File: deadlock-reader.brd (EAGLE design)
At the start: 49.2 x 49.5 mm, 49 parts, among them IC1 LM386M-1, IC2 STM32F072XX, IC3 MCP16301/H, IC4 MAX3232CSE, J1 RJ12 6p6c, X1 MINI-USB-SCHIELD-32005-301

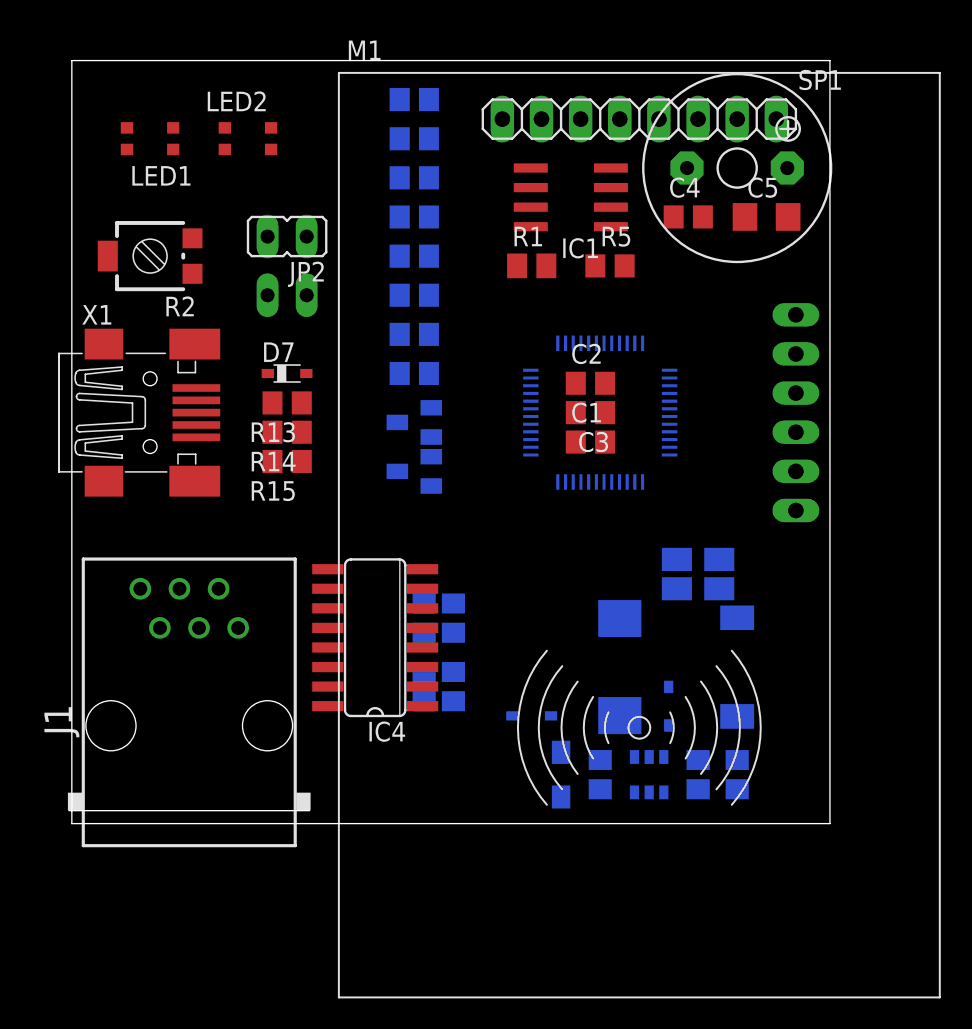
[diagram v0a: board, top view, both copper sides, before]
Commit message: [WIP] Route the power converter
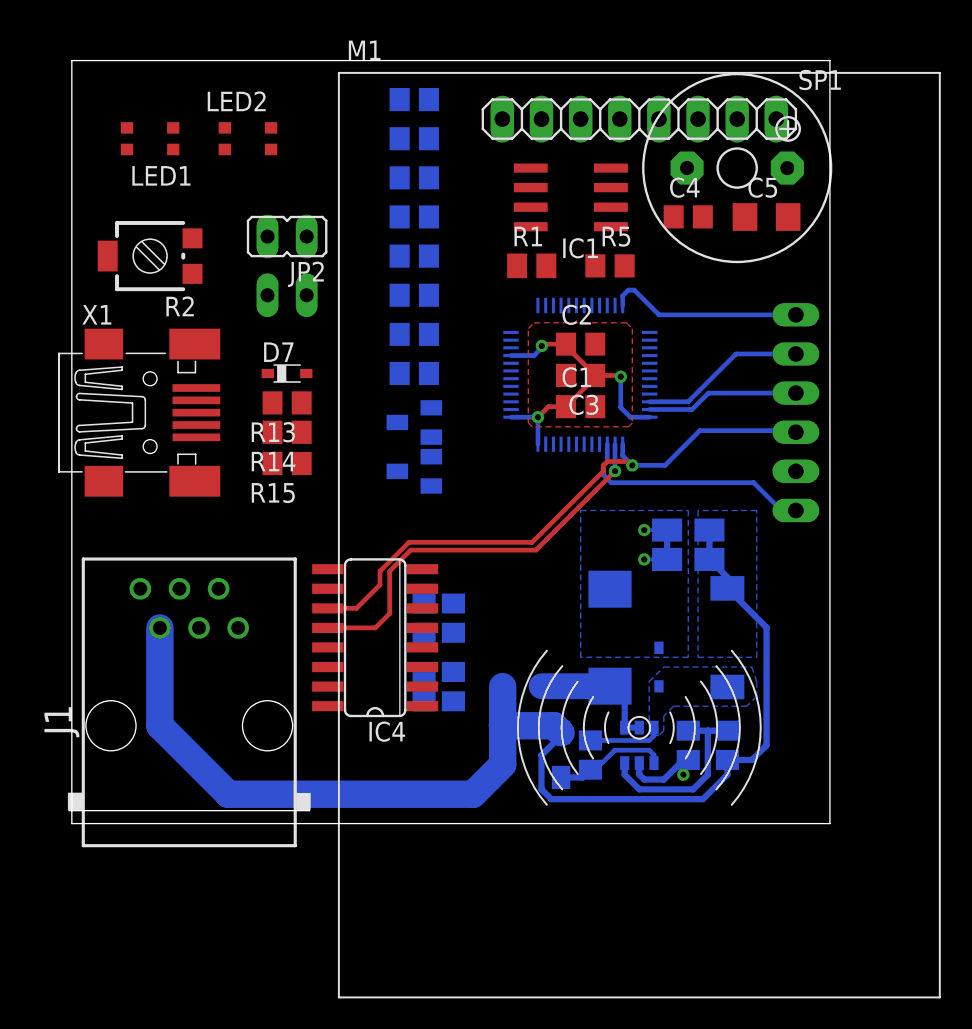
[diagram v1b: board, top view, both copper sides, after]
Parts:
- moved IC2 2.77 mm to (33.0, 29.1)
- moved D3 2.62 mm to (38.1, 10.2)
- moved C2 2.62 mm to (33.0, 31.1)
- moved C3 2.50 mm to (33.0, 29.1)
- moved C1 2.38 mm to (33.0, 27.1)
- moved IC3 2.01 mm to (36.8, 5.08)
- moved C6 2.01 mm to (34.9, 12.1)
- moved C9 2.01 mm to (40.0, 19.1)
- moved D5 2.01 mm to (29.2, 8.89)
- moved R11 2.01 mm to (42.5, 5.08), turned to 270 degrees
- moved R12 2.01 mm to (40.0, 5.08)
- moved C8 2.01 mm to (40.0, 17.1)
- moved L1 2.01 mm to (42.5, 12.1)
- moved C7 1.42 mm to (33.7, 4.45)
- moved D4 1.27 mm to (31.8, 4.45)
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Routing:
- net +3V3: track 0.00 -> 74.3 mm, vias 0 -> 3
- net RDR_TXD/SWDIO: track 0.00 -> 37.8 mm, vias 0 -> 1
- net N$9: track 0.00 -> 36.3 mm
- net RDR_RXD: track 0.00 -> 26.2 mm, vias 0 -> 1
- net GND: track 0.00 -> 20.6 mm, vias 0 -> 3
- net T_SWO: track 0.00 -> 15.5 mm
- net N$25: track 0.00 -> 12.3 mm
- net SWCLK: track 0.00 -> 10.8 mm
- net V+: track 0.00 -> 8.51 mm
- net N$23: track 0.00 -> 7.41 mm
- net N$22: track 0.00 -> 4.78 mm
- added copper zone on layer 16, net +3V3
- added copper zone on layer 1, net GND
- added copper zone on layer 16, net GND
- added copper zone on layer 16, net N$22
